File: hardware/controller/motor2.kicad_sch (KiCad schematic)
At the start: 55 parts, among them J10 Conn_01x01, J11 Conn_01x01, J12 Conn_01x09, J9 Conn_01x01, Q10 IPD90N04S4L04, Q11 IPD90N04S4L04, Q12 IPD90N04S4L04, Q13 IPD90N04S4L04, Q8 IPD90N04S4L04, Q9 IPD90N04S4L04, U14 MCP6541, U15 LM2105D, U16 MCP6541, U17 LM2105D, U18 MCP6541, U19 LM2105D

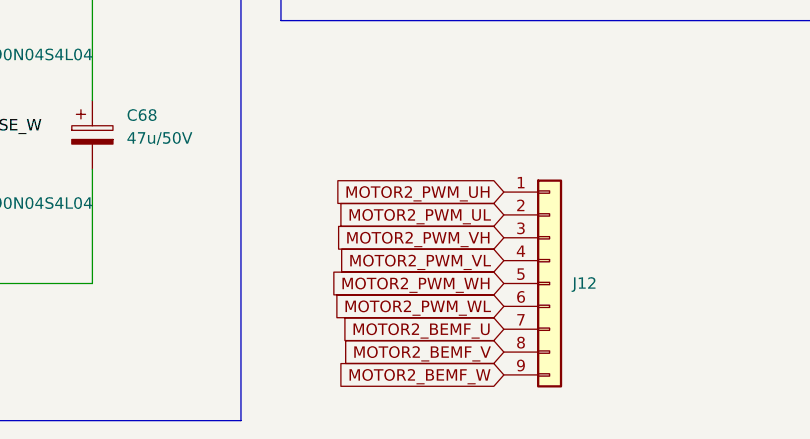
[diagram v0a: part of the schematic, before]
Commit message: wip routing power stages
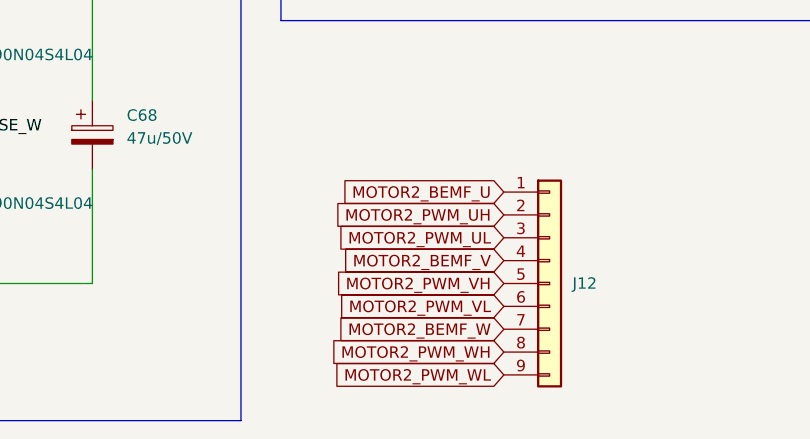
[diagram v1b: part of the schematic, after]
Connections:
- net MOTOR2_BEMF_U: now also J12.1 (Pin_1); no longer J12.7 (Pin_7)
- net MOTOR2_BEMF_V: now also J12.4 (Pin_4); no longer J12.8 (Pin_8)
- net MOTOR2_BEMF_W: now also J12.7 (Pin_7); no longer J12.9 (Pin_9)
- net MOTOR2_PWM_UH: now also J12.2 (Pin_2); no longer J12.1 (Pin_1)
- net MOTOR2_PWM_UL: now also J12.3 (Pin_3); no longer J12.2 (Pin_2)
- net MOTOR2_PWM_VH: now also J12.5 (Pin_5); no longer J12.3 (Pin_3)
- net MOTOR2_PWM_VL: now also J12.6 (Pin_6); no longer J12.4 (Pin_4)
- net MOTOR2_PWM_WH: now also J12.8 (Pin_8); no longer J12.5 (Pin_5)
- net MOTOR2_PWM_WL: now also J12.9 (Pin_9); no longer J12.6 (Pin_6)
